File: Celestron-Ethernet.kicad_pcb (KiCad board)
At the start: 4 copper layers, 88.9 x 31.8 mm, 73 parts, among them J1 USB_B_Micro, J2 RJ45_Abracon_ARJP11A-MASA-B-A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, J3 6P6C, SW1 SW_DIP_x02, U1 W5500, U2 ATmega32U4-AU, U3 LP2985-5.0, U4 LP2985-3.3, Y1 16MHz, Y2 25MHz

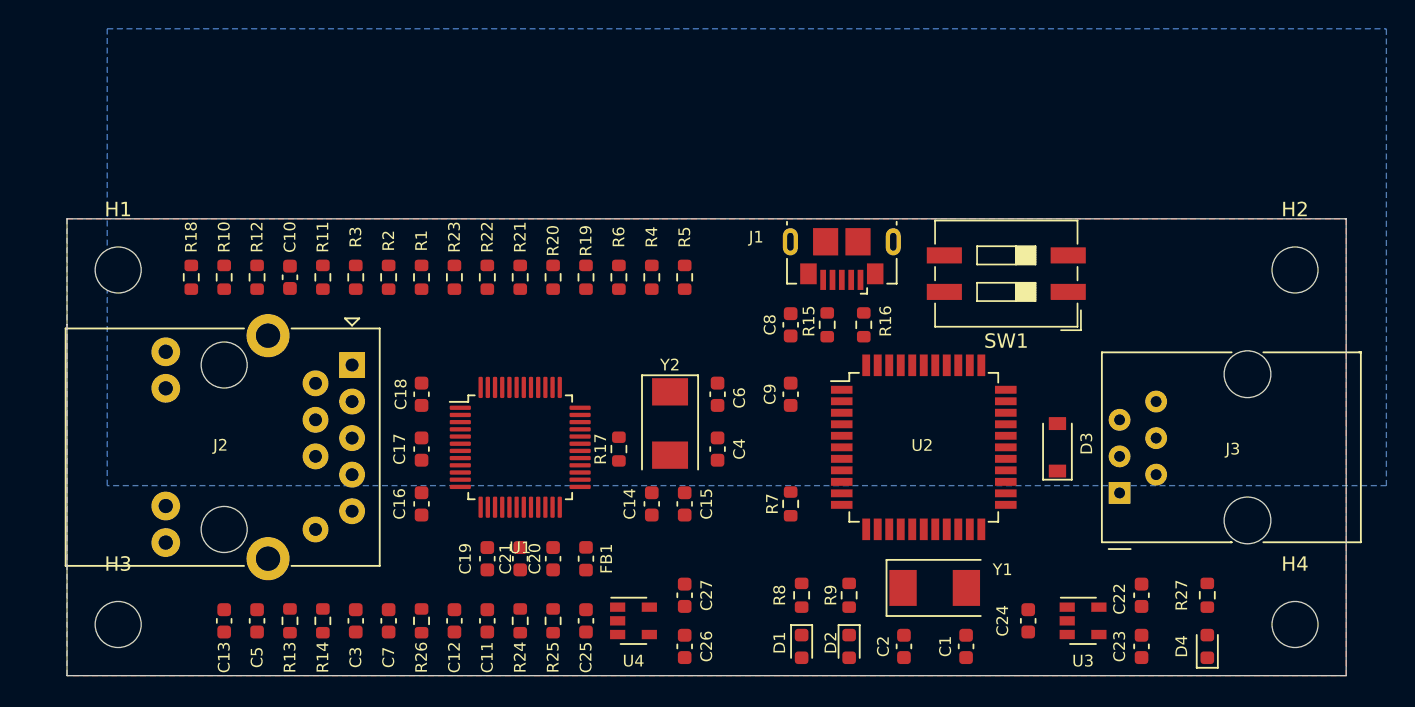
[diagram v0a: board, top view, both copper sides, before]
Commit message: traces complete
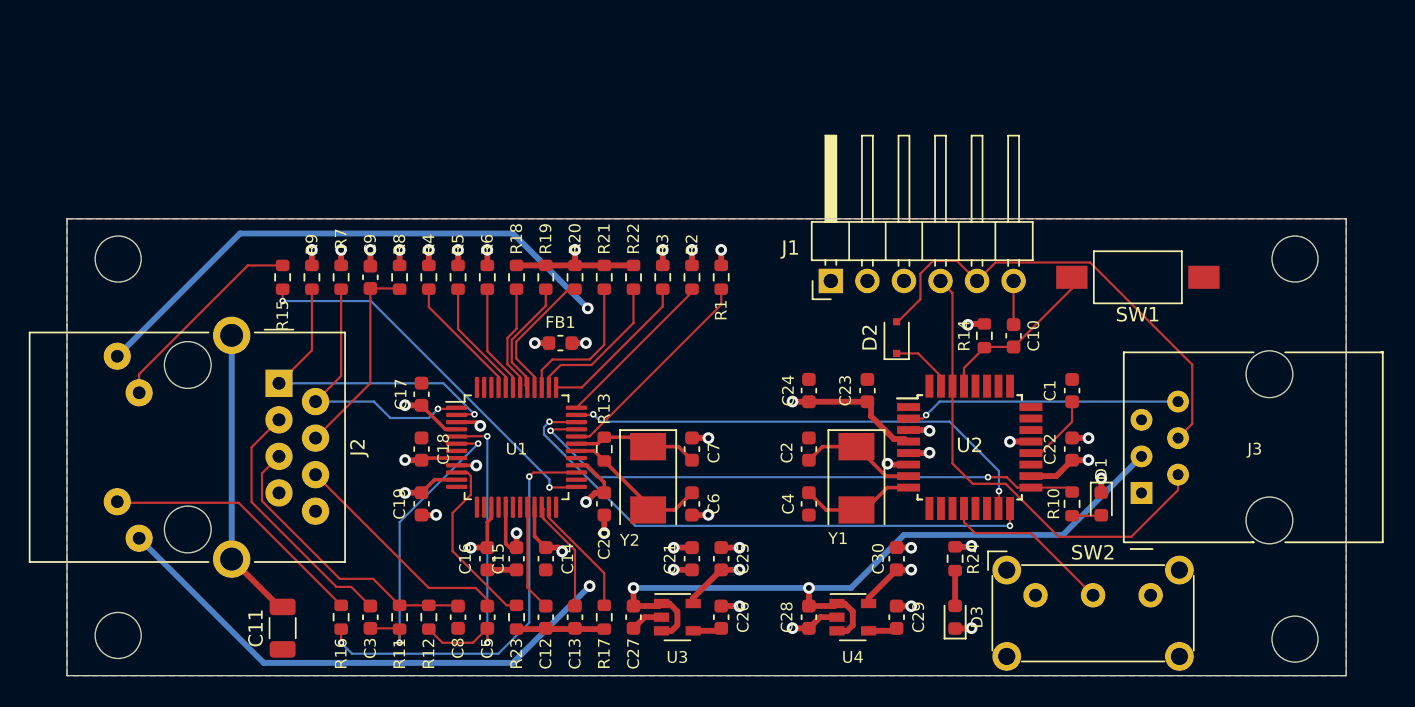
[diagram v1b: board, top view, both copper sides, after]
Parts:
- removed the C15 at (142.2, 102.4)
- removed the C25 at (137.7, 110.5)
- removed the C4 at (146.8, 98.6)
- removed the C9 at (151.9, 94.7)
- removed D4: Red, LED_SMD:LED_0603_1608Metric
- removed the R14 at (119.4, 110.5)
- removed the R15 at (154.4, 89.9)
- removed R25: 330R, Resistor_SMD:R_0603_1608Metric
- removed R26: 12.4K, Resistor_SMD:R_0603_1608Metric
- removed R27: 1K, Resistor_SMD:R_0603_1608Metric
- removed the R8 at (152.7, 108.7)
- removed the R9 at (156.0, 108.7)
- removed the U4 at (141.0, 110.5)
- added C1: 100nF, Capacitor_SMD:C_0603_1608Metric, F.Cu at (171.4, 94.5)
- added C10: 100nF, Capacitor_SMD:C_0603_1608Metric, F.Cu at (167.4, 90.7)
- added C20: 100nF, Capacitor_SMD:C_0603_1608Metric, F.Cu at (138.9, 102.4)
- added C22: 100nF, Capacitor_SMD:C_0603_1608Metric, F.Cu at (171.4, 98.6)
- added C23: 100nF, Capacitor_SMD:C_0603_1608Metric, F.Cu at (157.2, 94.5)
- added C27: 1uF, Capacitor_SMD:C_0603_1608Metric, F.Cu at (141.0, 110.2)
- added C28: 1uF, Capacitor_SMD:C_0603_1608Metric, F.Cu at (153.2, 110.2)
- added R10: 330R, Resistor_SMD:R_0603_1608Metric, F.Cu at (171.4, 102.4)
- added R11: 82R, Resistor_SMD:R_0603_1608Metric, F.Cu at (124.7, 110.2)
- added R12: 82R, Resistor_SMD:R_0603_1608Metric, F.Cu at (126.7, 110.2)
- added R23: 12.4K, Resistor_SMD:R_0603_1608Metric, F.Cu at (132.8, 110.2)
- added SW2: DHCP, Button_Switch_THT:SW_E-Switch_EG1224_SPDT_Angled, F.Cu at (168.9, 108.7)
- added U3: LP2985-3.3, Package_TO_SOT_SMD:SOT-23-5, F.Cu at (144.0, 110.2)
- C11: value 10nF -> 1nF/2KV; footprint Capacitor_SMD:C_0603_1608Metric -> Capacitor_SMD:C_1206_3216Metric
- C13: value 1nF/2KV -> 10nF
- C2: renamed from C1; value 22pF -> 18pF
- C24: value 1uF -> 10uF
- C3: value 10nF -> 6.8nF
- C4: renamed from C2; value 22pF -> 18pF
- C7: value 6.8nF -> 18pF
- C8: value 100nF -> 10nF
- D1: value Ylw -> Red
- D2: value Grn -> 1N4148W; footprint LED_SMD:LED_0603_1608Metric -> Diode_SMD:D_SOD-323F
- D3: value 1N4148W -> Red; footprint Diode_SMD:D_SOD-123 -> LED_SMD:LED_0603_1608Metric
- J1: value USB_B_Micro -> FTDI; footprint Connector_USB:USB_Micro-B_GCT_USB3076-30-A -> Connector_PinHeader_2.54mm:PinHeader_1x06_P2.54mm_Horizontal
- J2: value RJ45_Abracon_ARJP11A-MASA-B-A-EMU2 -> RJ45_Amphenol_RJMG1BD3B8K1ANR; footprint Connector_RJ:RJ45_Abracon_ARJP11A-MA_Horizontal -> Connector_RJ:RJ45_Amphenol_RJMG1BD3B8K1ANR
- R13: value 49R9 -> 1M
- R16: value 22R -> 330R
- R17: value 1M -> 10K
- R24: value 10K -> 1K
- SW1: value SW_DIP_x02 -> SW_Push; footprint Button_Switch_SMD:SW_DIP_SPSTx02_Slide_9.78x7.26mm_W8.61mm_P2.54mm -> Button_Switch_SMD:SW_SPST_FSMSM
- U2: value ATmega32U4-AU -> ATmega328-AU; footprint Package_QFP:TQFP-44_10x10mm_P0.8mm -> Package_QFP:TQFP-32_7x7mm_P0.8mm
- moved R16 41.6 mm to (120.7, 110.2)
- moved C8 30.8 mm to (128.8, 110.2)
- moved R24 30.5 mm to (163.3, 106.2)
- moved R13 24.9 mm to (138.9, 98.6)
- moved C13 24.4 mm to (136.9, 110.2)
- moved C7 24.2 mm to (145.0, 98.6)
- moved D1 23.1 mm to (173.5, 102.4)
- moved C24 22.1 mm to (153.2, 94.5), turned to 90 degrees
- moved D2 21.7 mm to (159.3, 90.8), turned to 90 degrees
- moved R14 17.8 mm to (165.4, 90.7)
- moved C2 17.5 mm to (153.2, 98.6), turned to 270 degrees
- moved C30 17.2 mm to (159.3, 106.2)
- moved C29 17.1 mm to (159.3, 110.2), turned to 90 degrees
- moved C5 16.0 mm to (130.8, 110.2)
- moved U4 16.0 mm to (156.2, 110.2)
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- renumbered C21 to C14, C20 to C15, C19 to C16, C18 to C17, C17 to C18, C16 to C19, C14 to C21, C27 to C25, C23 to C29, C22 to C30, C10 to C9, R6 to R1, R7 to R14, R18 to R15, R23 to R18, R22 to R19, R5 to R2, R21 to R20, R20 to R21, R19 to R22, R4 to R3, R3 to R4, R2 to R5, R1 to R6, R12 to R7, R11 to R8, R10 to R9, U3 to U4
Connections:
- C11 pad 2: Net-(C11-Pad2) -> GNDPWR
- C13 pad 2: GNDPWR -> Net-(C13-Pad2)
- C2 pad 2: Net-(C1-Pad2) -> Net-(C2-Pad2)
- C24 pad 1: /12V -> +5V
- C3 pad 1: GND -> Net-(C3-Pad1)
- C3 pad 2: Net-(C3-Pad2) -> /RD+
- C4 pad 2: Net-(C2-Pad2) -> Net-(C4-Pad2)
- C5 pad 1: Net-(C5-Pad1) -> /RD-
- C7 pad 1: Net-(C7-Pad1) -> GND
- C8 pad 1: Net-(C8-Pad1) -> GND
- C8 pad 2: GND -> /RCT
- C9 pad 2: Net-(C10-Pad2) -> /TCT
- D1 pad 1: Net-(D1-Pad1) -> GND
- D1 pad 2: +5V -> Net-(D1-Pad2)
- D2 pad 2: +5V -> /TXO
- D3 pad 1: Net-(D3-Pad1) -> GND
- J1 pad 1: /USB_PWR -> GND
- J1 pad 2: Net-(J1-Pad2) -> GND
- J1 pad 3: Net-(J1-Pad3) -> +5V
- J1 pad 4: Net-(J1-Pad4) -> /RXI
- J1 pad 5: GND -> /TXO
- J1 pad 6: Net-(J1-Pad6) -> /DTR
- J2 pad 13: +3V3 -> GNDPWR
- J3 pad 2: Net-(J3-Pad2) -> /RXI
- J3 pad 3: /12V -> +12V
- J3 pad 4: Net-(D3-Pad2) -> /TXO
- J3 pad 6: Net-(J3-Pad6) -> /D8
- R13 pad 1: Net-(C3-Pad2) -> Net-(C7-Pad2)
- R13 pad 2: Net-(C5-Pad1) -> Net-(C6-Pad2)
- R14 pad 2: Net-(R7-Pad2) -> Net-(C10-Pad1)
- R15 pad 1: Net-(J2-Pad12) -> /LEDG_K
- R16 pad 1: Net-(J1-Pad2) -> /LEDY_K
- R17 pad 1: Net-(C6-Pad2) -> Net-(R17-Pad1)
- R17 pad 2: Net-(C4-Pad2) -> GND
- R24 pad 1: Net-(R24-Pad1) -> +5V
- R24 pad 2: GND -> Net-(D3-Pad2)
- R7 pad 1: Net-(J2-Pad1) -> /TD-
- R7 pad 2: +3V3 -> +3.3VA
- R8 pad 1: Net-(C10-Pad2) -> /TCT
- R8 pad 2: +3V3 -> +3.3VA
- R9 pad 1: Net-(J2-Pad2) -> /TD+
- R9 pad 2: +3V3 -> +3.3VA
- SW1 pad 1: /USB_PWR -> GND
- SW1 pad 2: /DCHP_ENA -> Net-(C10-Pad1)
- U1 pad 1: Net-(J2-Pad2) -> /TD-
- U1 pad 2: Net-(J2-Pad1) -> /TD+
- U1 pad 22: Net-(C11-Pad2) -> Net-(C13-Pad2)
- U1 pad 23: Net-(R24-Pad1) -> Net-(R17-Pad1)
- U1 pad 27: Net-(R25-Pad2) -> Net-(R16-Pad2)
- U1 pad 30: Net-(C4-Pad2) -> Net-(C6-Pad2)
- U1 pad 31: Net-(C6-Pad2) -> Net-(C7-Pad2)
- U1 pad 33: Net-(U1-Pad33) -> /SCK
- U1 pad 34: Net-(U1-Pad34) -> /MISO
- U1 pad 35: Net-(U1-Pad35) -> /MOSI
- U1 pad 5: Net-(C5-Pad1) -> Net-(C5-Pad2)
- U1 pad 6: Net-(C7-Pad2) -> Net-(C3-Pad1)
- U2 pad 10: Net-(U1-Pad34) -> Net-(U2-Pad10)
- U2 pad 11: Net-(U1-Pad35) -> Net-(U2-Pad11)
- U2 pad 13: Net-(R7-Pad2) -> Net-(U2-Pad13)
- U2 pad 14: +5V -> Net-(U2-Pad14)
- U2 pad 15: GND -> /MOSI
- U2 pad 16: Net-(C2-Pad2) -> /MISO
- U2 pad 17: Net-(C1-Pad2) -> /SCK
- U2 pad 18: Net-(U2-Pad18) -> +5V
- U2 pad 2: +5V -> /D8
- U2 pad 20: Net-(J3-Pad2) -> Net-(C1-Pad2)
- U2 pad 21: Net-(D3-Pad1) -> GND
- U2 pad 23: GND -> Net-(U2-Pad23)
- U2 pad 24: +5V -> Net-(U2-Pad24)
- U2 pad 25: Net-(J3-Pad6) -> Net-(U2-Pad25)
- U2 pad 28: /DCHP_ENA -> Net-(U2-Pad28)
- U2 pad 29: Net-(U2-Pad29) -> Net-(C10-Pad1)
- U2 pad 3: Net-(R16-Pad2) -> GND
- U2 pad 30: Net-(U2-Pad30) -> /RXI
- U2 pad 31: Net-(U2-Pad31) -> Net-(D2-Pad1)
- U2 pad 4: Net-(R15-Pad1) -> +5V
- U2 pad 6: Net-(C9-Pad1) -> +5V
- U2 pad 7: +5V -> Net-(C2-Pad2)
- U2 pad 8: Net-(R8-Pad1) -> Net-(C4-Pad2)
- U2 pad 9: Net-(U1-Pad33) -> Net-(U2-Pad9)
- U4 pad 1: /12V -> +12V
- U4 pad 3: /12V -> +12V
- Y1 pad 2: Net-(C1-Pad2) -> Net-(C4-Pad2)
- Y2 pad 1: Net-(C6-Pad2) -> Net-(C7-Pad2)
- Y2 pad 2: Net-(C4-Pad2) -> Net-(C6-Pad2)
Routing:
- net +3V3: track 0.00 -> 93.5 mm, vias 0 -> 12
- net +12V: track 0.00 -> 52.7 mm, vias 0 -> 2
- net GND: track 0.00 -> 45.4 mm, vias 0 -> 20
- net /SCK: track 0.00 -> 39.9 mm, vias 0 -> 2
- net /MISO: track 0.00 -> 39.2 mm, vias 0 -> 2
- net /MOSI: track 0.00 -> 33.6 mm, vias 0 -> 2
- net /RXI: track 0.00 -> 33.2 mm
- net /TXO: track 0.00 -> 32.9 mm
- net +3.3VA: track 0.00 -> 29.0 mm, vias 0 -> 10
- net Net-(R16-Pad2): track 0.00 -> 28.8 mm, vias 0 -> 2
- net Net-(R15-Pad2): track 0.00 -> 26.9 mm, vias 0 -> 2
- net /TD+: track 0.00 -> 23.2 mm, vias 0 -> 1
- net Net-(C5-Pad2): track 0.00 -> 22.4 mm, vias 0 -> 2
- net +5V: track 0.00 -> 22.1 mm, vias 0 -> 6
- net GNDPWR: track 0.00 -> 20.5 mm
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- added copper zone on In2.Cu, net +3.3VA
